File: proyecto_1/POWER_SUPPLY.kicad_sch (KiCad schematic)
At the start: 7 parts, among them U14 B0505S-W2R2, U15 fuse_CC12H1.5A-TR

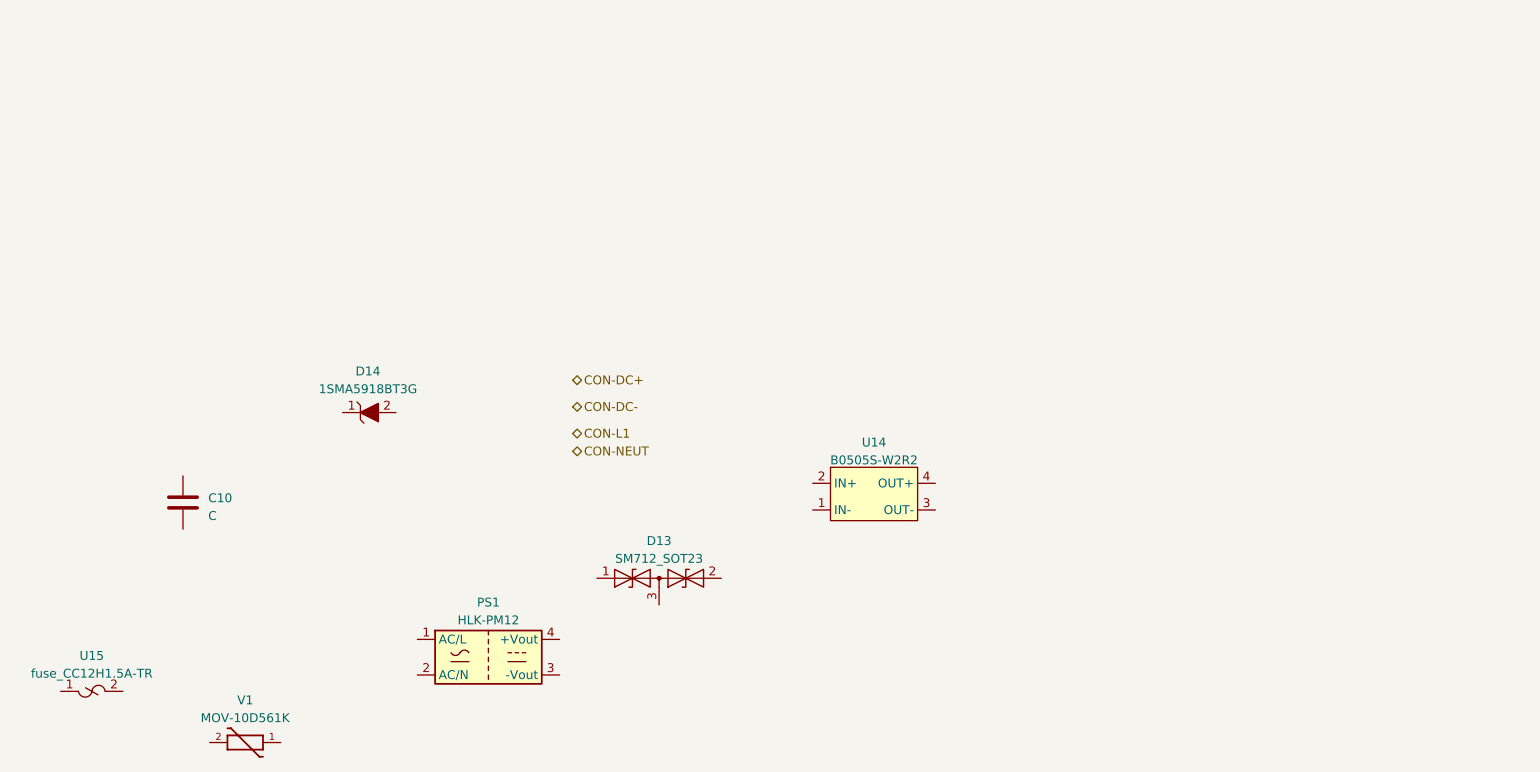
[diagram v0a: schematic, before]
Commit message: fuente
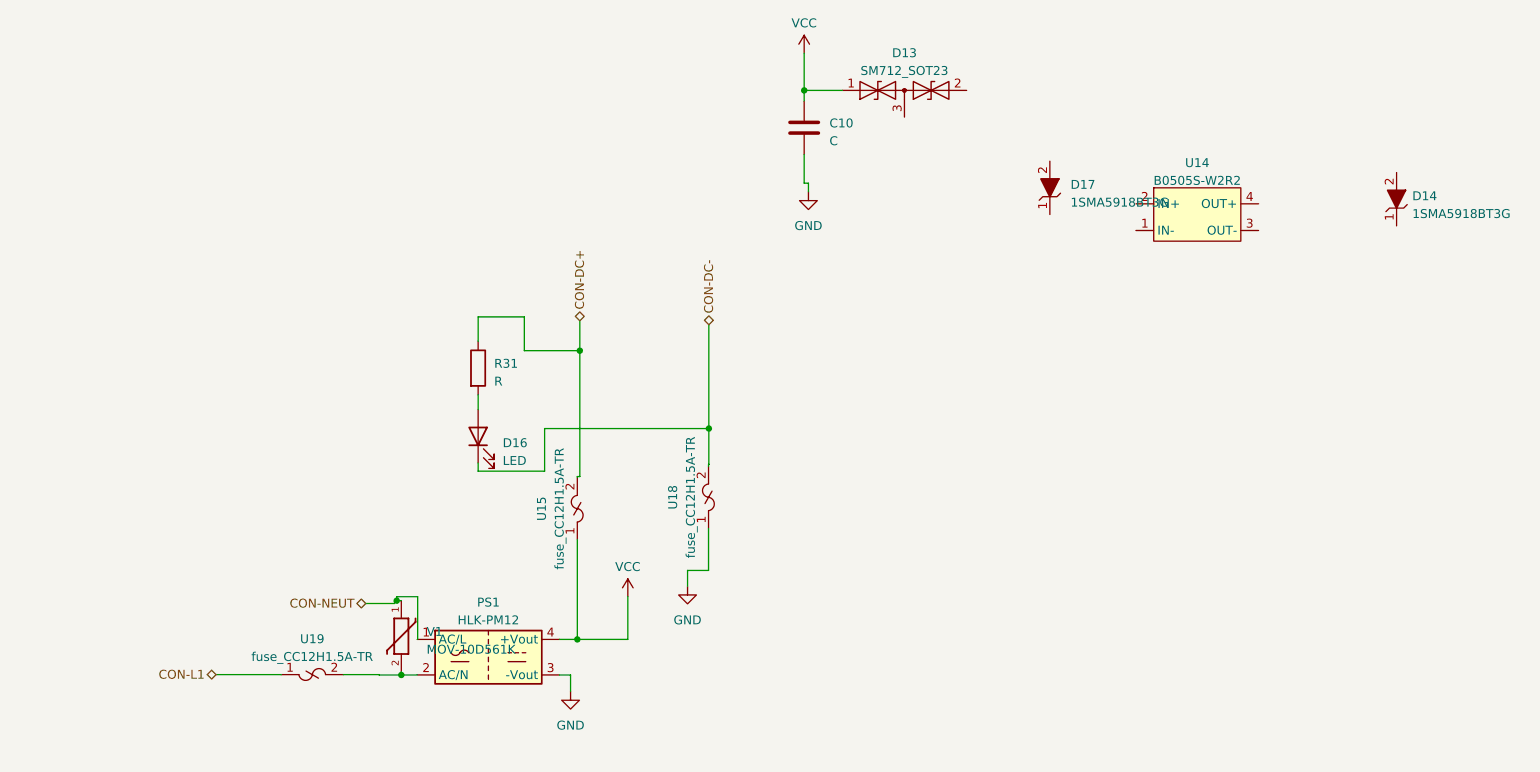
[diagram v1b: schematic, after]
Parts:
- added D16: LED, symbol Device:LED
- added D17: 1SMA5918BT3G, Diode_SMD:D_SMB, symbol nuevo simbolos:1SMA5918BT3G
- added R31: R, symbol Device:R
- added U18, U19: fuse_CC12H1.5A-TR, nuevo simbolo:CC12H1.5A-TR, symbol nuevo simbolos:fuse_CC12H1.5A-TR
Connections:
- net CON-DC+: now also U15.2, R31.1
- net CON-DC-: now also D16.1 (K), U18.2
- net CON-L1: now also U19.1
- net CON-NEUT: now also PS1.1 (AC/L), V1.1
- net VCC: now reaches U15.1
- net VCC: now also C10.1, D13.1 (A1), PS1.4 (+Vout)
- net at PS1.2 (AC/N): now also V1.2, U19.2
- net GND: now reaches PS1.3 (-Vout)
- net GND: now also C10.2, U18.1
- new net: D16.2 (A), R31.2
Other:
- moved on the sheet: C10, D13, D14, U14, U15, V1
